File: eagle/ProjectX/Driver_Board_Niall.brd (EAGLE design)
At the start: 100 x 100 mm, 185 parts, among them IC2 NCV78M05BDTRKG, J1 694102303002, U1 TC4427AEOA, U10 TC4427AEOA, U11 TC4427AEOA, U12 TC4427AEOA, U1200 CD74HC4067SM96, U13 TC4427AEOA, U14 TC4427AEOA, U15 TC4427AEOA, U16 TC4427AEOA, U17 TC4427AEOA, U18 TC4427AEOA, U19 TC4427AEOA, U2 TC4427AEOA, U20 TC4427AEOA, U200 ADA4091-2ARZ-RL, U21 TC4427AEOA, U22 TC4427AEOA, U23 TC4427AEOA, U24 TC4427AEOA, U25 TC4427AEOA, U26 TC4427AEOA, U27 TC4427AEOA, U28 TC4427AEOA, U29 TC4427AEOA, U3 TC4427AEOA, U30 TC4427AEOA, U31 TC4427AEOA, U32 TC4427AEOA, U33 TC4427AEOA, U34 TC4427AEOA, U35 TC4427AEOA, U36 TC4427AEOA, U37 TC4427AEOA, U38 TC4427AEOA, U39 TC4427AEOA, U4 TC4427AEOA, U40 TC4427AEOA, U41 TC4427AEOA, U42 TC4427AEOA, U43 TC4427AEOA, U44 TC4427AEOA, U45 TC4427AEOA, U46 TC4427AEOA, U47 TC4427AEOA, U48 TC4427AEOA, U49 TC4427AEOA, U5 TC4427AEOA, U50 TC4427AEOA, U6 TC4427AEOA, U7 TC4427AEOA, U8 TC4427AEOA, U9 TC4427AEOA

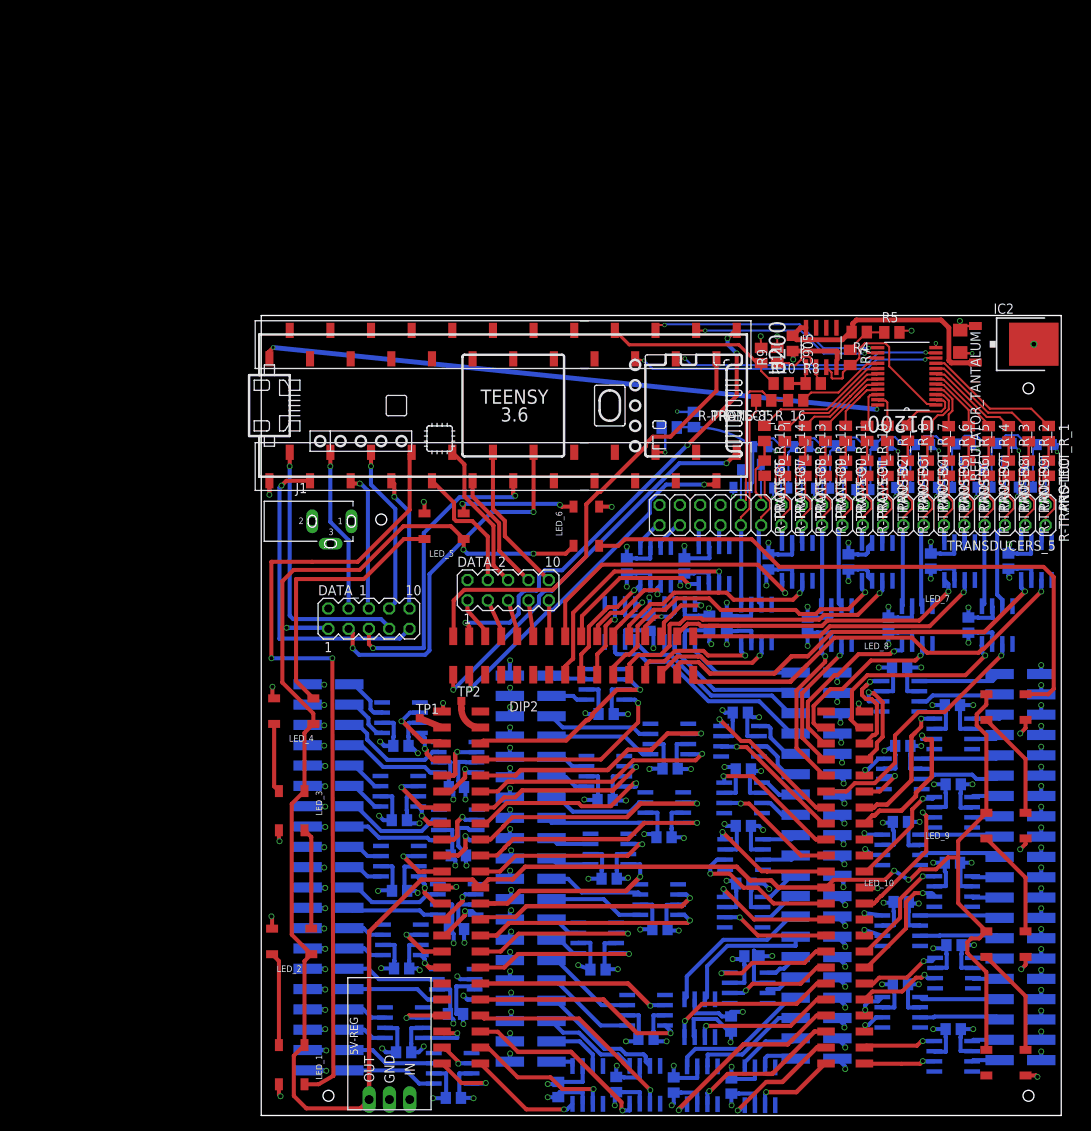
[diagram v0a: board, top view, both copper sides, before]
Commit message: Niall Boards new layout that should slot together
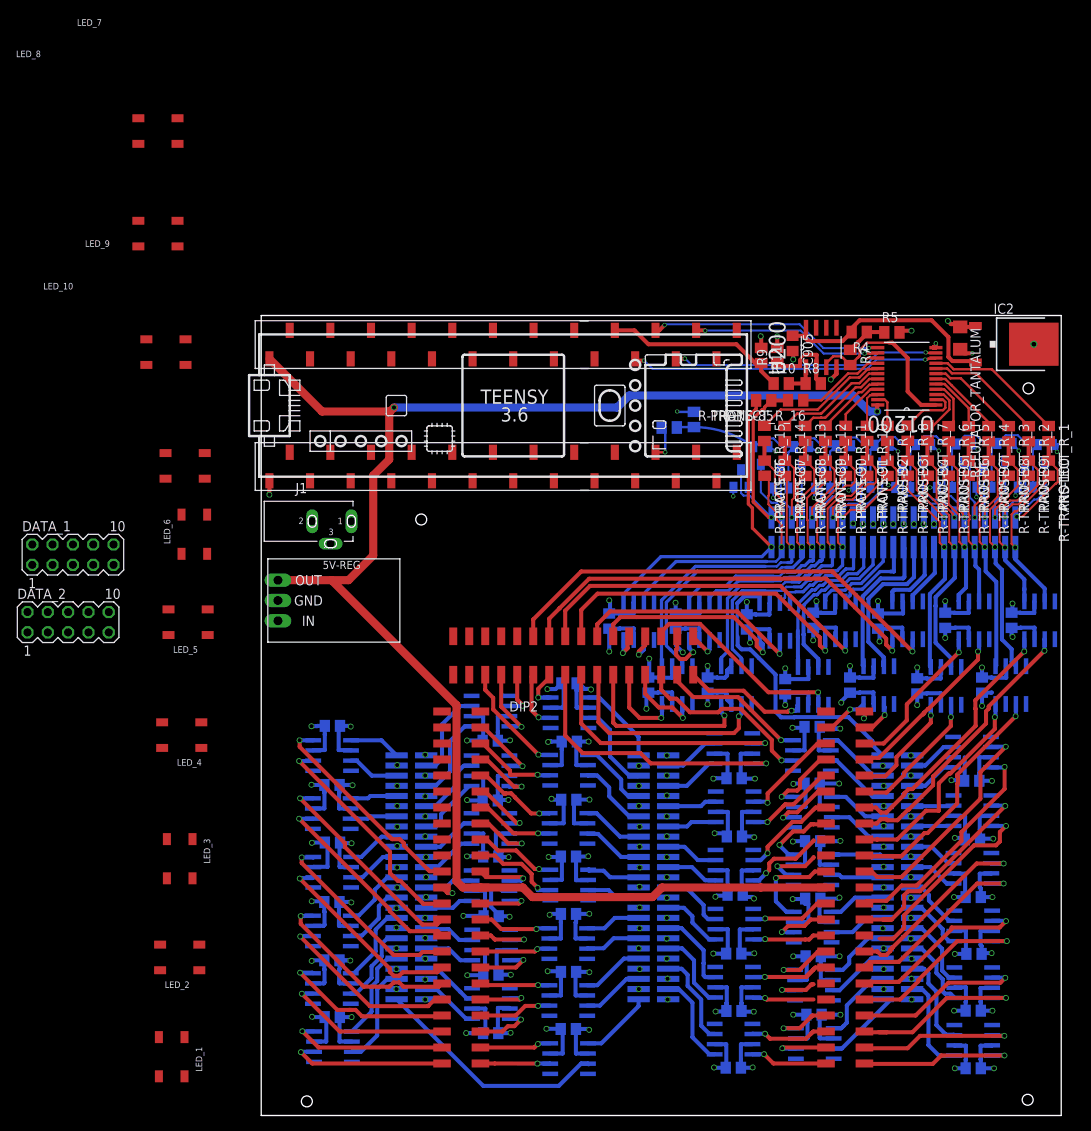
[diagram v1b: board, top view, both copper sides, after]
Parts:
- removed TP1, TP2: TPSTP10SQ, testpad:TP10SQ
- removed TRANSDUCERS_1, TRANSDUCERS_2, TRANSDUCERS_3, TRANSDUCERS_4: 40_PIN_SMD, Parts:40_PIN_SMD
- removed TRANSDUCERS_5: (no value), pinhead:2X20
- added 1, 2, 3, 4: PHB_1MM27_2X25_SNS, _hhn_con_pinhead_box_1mm27:PHB_1MM27_2X25_SNS
- moved LED_8 129.3 mm to (-12.9, 110.2)
- moved LED_9 128.5 mm to (-11.9, 95.4)
- moved LED_7 128.1 mm to (-12.9, 123.1)
- moved LED_10 126.9 mm to (-9.51, 81.2)
- moved 5V-REG 63.9 mm to (2.09, 64.4), turned to 270 degrees
- moved U40 56.3 mm to (72.4, 61.9), turned to 90 degrees
- moved DATA_2 55.1 mm to (-24.1, 61.7)
- moved C40 54.0 mm to (69.0, 61.9), turned to 90 degrees
- moved C12 50.5 mm to (38.5, 54.0), turned to 180 degrees
- moved U38 49.3 mm to (64.2, 61.7), turned to 90 degrees
- moved LED_6 49.0 mm to (-8.36, 72.7)
- moved C38 48.0 mm to (60.7, 61.7), turned to 90 degrees
- moved U12 47.5 mm to (38.5, 50.3), turned to 180 degrees
- moved U20 47.0 mm to (38.5, 7.11), turned to 180 degrees
- moved C29 44.9 mm to (38.5, 46.7), turned to 180 degrees
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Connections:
- removed net N$23: DIP2.8, TP1.TP
- removed net N$24: DIP2.9, TP2.TP
- removed net N$25: DATA_2.9, DIP2.190
- removed net N$26: DATA_2.7, DIP2.193
- removed net N$27: DATA_2.5, DIP2.197
- removed net N$28: DATA_2.1, DIP2.203
- removed net N$29: DATA_2.3, DIP2.200
- net +5V: no longer DATA_1.1
- net 1: now also DIP2.75; no longer DIP2.77
- net 10: now also DIP2.47; no longer DIP2.41
- net 100: now also DIP2.137; no longer DIP2.162
- net 11: now also DIP2.48; no longer DIP2.39
- net 12: now also DIP2.50; no longer DIP2.35
- net 13: now also DIP2.40; no longer DIP2.33
- net 14: now also DIP2.36; no longer DIP2.30
- net 15: now also DIP2.60; no longer DIP2.28
- net 16: now also DIP2.62; no longer DIP2.24
- net 17: now also DIP2.29; no longer DIP2.22
- net 18: now also DIP2.23; no longer DIP2.18
- net 19: now also DIP2.64; no longer DIP2.15
- net 2: now also DIP2.77; no longer DIP2.75
- net 20: now also DIP2.69; no longer DIP2.11
- net 21: now also DIP2.19; no longer DIP2.82
- net 22: now also DIP2.25; no longer DIP2.76
- net 23: now also DIP2.192; no longer DIP2.74
- net 24: now also DIP2.196; no longer DIP2.65
- net 25: now also DIP2.102; no longer DIP2.63
- net 26: now also DIP2.109; no longer DIP2.61
- net 27: now also DIP2.31; no longer DIP2.55
- net 28: now also DIP2.34; no longer DIP2.49
- net 29: now also DIP2.133; no longer DIP2.47
- net 3: now also DIP2.35; no longer DIP2.69
- net 30: now also DIP2.138; no longer DIP2.42
- net 31: now also DIP2.42; no longer DIP2.40
- net 32: now also DIP2.49; no longer DIP2.36
- net 33: now also DIP2.145; no longer DIP2.34
- net 34: now also DIP2.151; no longer DIP2.31
- net 35: now also DIP2.61; no longer DIP2.29
- net 36: now also DIP2.65; no longer DIP2.25
- net 37: now also DIP2.189; no longer DIP2.23
- net 38: now also DIP2.186; no longer DIP2.19
- net 39: now also DIP2.76; no longer DIP2.16
- net 4: now also DIP2.39; no longer DIP2.64
- net 40: now also DIP2.82; no longer DIP2.12
- net 41: now also DIP2.16; no longer DIP2.165
- net 42: now also DIP2.9; no longer DIP2.168
- net 43: now also DIP2.202; no longer DIP2.178
- net 44: now also DIP2.199; no longer DIP2.181
- net 45: now also DIP2.126; no longer DIP2.138
- net 46: now also DIP2.128; no longer DIP2.135
- net 47: now also DIP2.164; no longer DIP2.133
- net 48: now also DIP2.167; no longer DIP2.129
- net 49: now also DIP2.147; no longer DIP2.127
- net 5: now also DIP2.74; no longer DIP2.62
- net 50: now also DIP2.140; no longer DIP2.123
- net 51: now also DIP2.135; no longer DIP2.120
- net 52: now also DIP2.129; no longer DIP2.116
- net 53: now also DIP2.116; no longer DIP2.107
- net 54: now also DIP2.123; no longer DIP2.102
- net 55: now also DIP2.127; no longer DIP2.113
- net 56: now also DIP2.120; no longer DIP2.109
- net 57: now also DIP2.205; no longer DIP2.99
- net 58: now also DIP2.12; no longer DIP2.97
- net 59: now also DIP2.90; no longer DIP2.94
- net 6: now also DIP2.63; no longer DIP2.60
- net 60: now also DIP2.97; no longer DIP2.90
- net 61: now also DIP2.99; no longer DIP2.152
- net 62: now also DIP2.94; no longer DIP2.150
- net 63: now also DIP2.113; no longer DIP2.139
- net 64: now also DIP2.107; no longer DIP2.137
- net 65: now also DIP2.93; no longer DIP2.146
- net 66: now also DIP2.96; no longer DIP2.144
- net 67: now also DIP2.98; no longer DIP2.128
- net 68: now also DIP2.100; no longer DIP2.126
- net 69: now also DIP2.106; no longer DIP2.134
- net 7: now also DIP2.41; no longer DIP2.50
- net 70: now also DIP2.108; no longer DIP2.132
- net 71: now also DIP2.112; no longer DIP2.115
- net 72: now also DIP2.115; no longer DIP2.112
- net 73: now also DIP2.119; no longer DIP2.122
- net 74: now also DIP2.122; no longer DIP2.119
- net 75: now also DIP2.178; no longer DIP2.108
- net 76: now also DIP2.180; no longer DIP2.106
- net 77: now also DIP2.162; no longer DIP2.100
- net 78: now also DIP2.165; no longer DIP2.98
- net 79: now also DIP2.185; no longer DIP2.96
- net 8: now also DIP2.45; no longer DIP2.48
- net 80: now also DIP2.187; no longer DIP2.93
- net 81: now also DIP2.153; no longer DIP2.186
- net 82: now also DIP2.160; no longer DIP2.180
- net 83: now also DIP2.190; no longer DIP2.185
- net 84: now also DIP2.193; no longer DIP2.189
- net 85: now also DIP2.172; no longer DIP2.171
- net 86: now also DIP2.168; no longer DIP2.167
- net 87: now also DIP2.177; no longer DIP2.187
- net 88: now also DIP2.171; no longer DIP2.172
- net 89: now also DIP2.163; no longer DIP2.145
- net 9: now also DIP2.55; no longer DIP2.45
- net 90: now also DIP2.161; no longer DIP2.147
- net 92: now also DIP2.181; no longer DIP2.177
- net 93: now also DIP2.146; no longer DIP2.151
- net 94: now also DIP2.144; no longer DIP2.153
- net 95: now also DIP2.152; no longer DIP2.163
- net 96: now also DIP2.150; no longer DIP2.161
- net 97: now also DIP2.134; no longer DIP2.160
- net 98: now also DIP2.132; no longer DIP2.140
- net 99: now also DIP2.139; no longer DIP2.164
- net FROM_TRANS_100: now also 1.2; no longer TRANSDUCERS_5.1
- net FROM_TRANS_85: now also 1.50; no longer TRANSDUCERS_5.31
- net FROM_TRANS_86: now also 1.48; no longer TRANSDUCERS_5.29
- net FROM_TRANS_87: now also 1.46; no longer TRANSDUCERS_5.27
- net FROM_TRANS_88: now also 1.44; no longer TRANSDUCERS_5.25
- net FROM_TRANS_89: now also 1.42; no longer TRANSDUCERS_5.23
- net FROM_TRANS_90: now also 1.40; no longer TRANSDUCERS_5.21
- net FROM_TRANS_91: now also 1.38; no longer TRANSDUCERS_5.19
- net FROM_TRANS_92: now also 1.36; no longer TRANSDUCERS_5.17
- net FROM_TRANS_93: now also 1.16; no longer TRANSDUCERS_5.15
- net FROM_TRANS_94: now also 1.14; no longer TRANSDUCERS_5.13
- net FROM_TRANS_95: now also 1.12; no longer TRANSDUCERS_5.11
- net FROM_TRANS_96: now also 1.10; no longer TRANSDUCERS_5.9
- net FROM_TRANS_97: now also 1.8; no longer TRANSDUCERS_5.7
- net FROM_TRANS_98: now also 1.6; no longer TRANSDUCERS_5.5
- net FROM_TRANS_99: now also 1.4; no longer TRANSDUCERS_5.3
- net GND: now also 1.18, 1.20, 1.22, 1.24, 1.26, 1.28, 1.30, 1.32, 1.34, 2.10, 2.11, 2.14, 2.15, 2.18, 2.19, 2.2, 2.22, 2.23, 2.26, 2.27, 2.3, 2.30, 2.31, 2.34, 2.35, 2.38, 2.39, 2.42, 2.43, 2.46, 2.47, 2.50, 2.6, 2.7, 3.10, 3.11, 3.14, 3.15, 3.18, 3.19, 3.2, 3.22, 3.23, 3.26, 3.27, 3.3, 3.30, 3.31, 3.34, 3.35, 3.38, 3.39, 3.42, 3.43, 3.46, 3.47, 3.50, 3.6, 3.7, 4.10, 4.11, 4.14, 4.15, 4.18, 4.19, 4.2, 4.22, 4.23, 4.26, 4.27, 4.3, 4.30, 4.31, 4.34, 4.35, 4.38, 4.39, 4.42, 4.43, 4.46, 4.47, 4.50, 4.6, 4.7; no longer DATA_1.2, DATA_2.2, TRANSDUCERS_1.1, TRANSDUCERS_1.11, TRANSDUCERS_1.13, TRANSDUCERS_1.15, TRANSDUCERS_1.17, TRANSDUCERS_1.19, TRANSDUCERS_1.21, TRANSDUCERS_1.23, TRANSDUCERS_1.25, TRANSDUCERS_1.27, TRANSDUCERS_1.29, TRANSDUCERS_1.3, TRANSDUCERS_1.31, TRANSDUCERS_1.33, TRANSDUCERS_1.35, TRANSDUCERS_1.37, TRANSDUCERS_1.39, TRANSDUCERS_1.5, TRANSDUCERS_1.7, TRANSDUCERS_1.9, TRANSDUCERS_2.1, TRANSDUCERS_2.11, TRANSDUCERS_2.13, TRANSDUCERS_2.15, TRANSDUCERS_2.17, TRANSDUCERS_2.19, TRANSDUCERS_2.21, TRANSDUCERS_2.23, TRANSDUCERS_2.25, TRANSDUCERS_2.27, TRANSDUCERS_2.29, TRANSDUCERS_2.3, TRANSDUCERS_2.31, TRANSDUCERS_2.33, TRANSDUCERS_2.35, TRANSDUCERS_2.37, TRANSDUCERS_2.39, TRANSDUCERS_2.5, TRANSDUCERS_2.7, TRANSDUCERS_2.9, TRANSDUCERS_3.1, TRANSDUCERS_3.11, TRANSDUCERS_3.13, TRANSDUCERS_3.15, TRANSDUCERS_3.17, TRANSDUCERS_3.19, TRANSDUCERS_3.21, TRANSDUCERS_3.23, TRANSDUCERS_3.25, TRANSDUCERS_3.27, TRANSDUCERS_3.29, TRANSDUCERS_3.3, TRANSDUCERS_3.31, TRANSDUCERS_3.33, TRANSDUCERS_3.35, TRANSDUCERS_3.37, TRANSDUCERS_3.39, TRANSDUCERS_3.5, TRANSDUCERS_3.7, TRANSDUCERS_3.9, TRANSDUCERS_4.1, TRANSDUCERS_4.11, TRANSDUCERS_4.13, TRANSDUCERS_4.15, TRANSDUCERS_4.17, TRANSDUCERS_4.19, TRANSDUCERS_4.21, TRANSDUCERS_4.23, TRANSDUCERS_4.25, TRANSDUCERS_4.27, TRANSDUCERS_4.29, TRANSDUCERS_4.3, TRANSDUCERS_4.31, TRANSDUCERS_4.33, TRANSDUCERS_4.35, TRANSDUCERS_4.37, TRANSDUCERS_4.39, TRANSDUCERS_4.5, TRANSDUCERS_4.7, TRANSDUCERS_4.9, TRANSDUCERS_5.33, TRANSDUCERS_5.35, TRANSDUCERS_5.37, TRANSDUCERS_5.39
- net TEENSY_DATA_0: no longer DATA_1.7
- net TEENSY_DATA_1: no longer DATA_1.9
- net TEENSY_DATA_10: no longer DATA_2.10
- net TEENSY_DATA_11: no longer DATA_1.5
- net TEENSY_DATA_12: no longer DATA_1.3
- net TEENSY_DATA_2: no longer DATA_1.4
- net TEENSY_DATA_3: no longer DATA_1.6
- net TEENSY_DATA_31: no longer DIP2.3
- net TEENSY_DATA_32: no longer DIP2.5
- net TEENSY_DATA_33: no longer DIP2.2
- net TEENSY_DATA_34: no longer DIP2.4
- net TEENSY_DATA_4: no longer DATA_1.8
- net TEENSY_DATA_5: no longer DATA_1.10
- net TEENSY_DATA_7: no longer DATA_2.4
- net TEENSY_DATA_8: no longer DATA_2.6
- net TEENSY_DATA_9: no longer DATA_2.8
- net TO_TRAN_1: now also 4.9; no longer TRANSDUCERS_1.2
- net TO_TRAN_10: now also 4.16; no longer TRANSDUCERS_1.20
- net TO_TRAN_100: now also 1.1; no longer TRANSDUCERS_5.2
- net TO_TRAN_11: now also 4.33; no longer TRANSDUCERS_1.22
- net TO_TRAN_12: now also 4.29; no longer TRANSDUCERS_1.24
- net TO_TRAN_13: now also 4.20; no longer TRANSDUCERS_1.26
- net TO_TRAN_14: now also 4.24; no longer TRANSDUCERS_1.28
- net TO_TRAN_15: now also 4.25; no longer TRANSDUCERS_1.30
- net TO_TRAN_16: now also 4.21; no longer TRANSDUCERS_1.32
- net TO_TRAN_17: now also 4.28; no longer TRANSDUCERS_1.34
- net TO_TRAN_18: now also 4.32; no longer TRANSDUCERS_1.36
- net TO_TRAN_19: now also 4.17; no longer TRANSDUCERS_1.38
- net TO_TRAN_2: now also 4.5; no longer TRANSDUCERS_1.4
- net TO_TRAN_20: now also 4.13; no longer TRANSDUCERS_1.40
- net TO_TRAN_21: now also 3.33; no longer TRANSDUCERS_2.2
- net TO_TRAN_22: now also 3.29; no longer TRANSDUCERS_2.4
- net TO_TRAN_23: now also 3.49; no longer TRANSDUCERS_2.6
- net TO_TRAN_24: now also 3.45; no longer TRANSDUCERS_2.8
- net TO_TRAN_25: now also 3.12; no longer TRANSDUCERS_2.10
- net TO_TRAN_26: now also 3.16; no longer TRANSDUCERS_2.12
- net TO_TRAN_27: now also 3.25; no longer TRANSDUCERS_2.14
- net TO_TRAN_28: now also 3.21; no longer TRANSDUCERS_2.16
- net TO_TRAN_29: now also 3.28; no longer TRANSDUCERS_2.18
- net TO_TRAN_3: now also 4.49; no longer TRANSDUCERS_1.6
- net TO_TRAN_30: now also 3.32; no longer TRANSDUCERS_2.20
- net TO_TRAN_31: now also 3.17; no longer TRANSDUCERS_2.22
- net TO_TRAN_32: now also 3.13; no longer TRANSDUCERS_2.24
- net TO_TRAN_33: now also 3.36; no longer TRANSDUCERS_2.26
- net TO_TRAN_34: now also 3.40; no longer TRANSDUCERS_2.28
- net TO_TRAN_35: now also 3.9; no longer TRANSDUCERS_2.30
- net TO_TRAN_36: now also 3.5; no longer TRANSDUCERS_2.32
- net TO_TRAN_37: now also 3.44; no longer TRANSDUCERS_2.34
- net TO_TRAN_38: now also 3.48; no longer TRANSDUCERS_2.36
- net TO_TRAN_39: now also 3.1; no longer TRANSDUCERS_2.38
- net TO_TRAN_4: now also 4.45; no longer TRANSDUCERS_1.8
- net TO_TRAN_40: now also 4.1; no longer TRANSDUCERS_2.40
- net TO_TRAN_41: now also 4.36; no longer TRANSDUCERS_3.2
- net TO_TRAN_42: now also 4.40; no longer TRANSDUCERS_3.4
- net TO_TRAN_43: now also 4.44; no longer TRANSDUCERS_3.6
- net TO_TRAN_44: now also 4.48; no longer TRANSDUCERS_3.8
- net TO_TRAN_45: now also 2.44; no longer TRANSDUCERS_3.10
- net TO_TRAN_46: now also 2.48; no longer TRANSDUCERS_3.12
- net TO_TRAN_47: now also 2.45; no longer TRANSDUCERS_3.14
- net TO_TRAN_48: now also 2.41; no longer TRANSDUCERS_3.16
- net TO_TRAN_49: now also 2.37; no longer TRANSDUCERS_3.18
- net TO_TRAN_5: now also 4.4; no longer TRANSDUCERS_1.10
- net TO_TRAN_50: now also 2.33; no longer TRANSDUCERS_3.20
- net TO_TRAN_51: now also 2.29; no longer TRANSDUCERS_3.22
- net TO_TRAN_52: now also 2.25; no longer TRANSDUCERS_3.24
- net TO_TRAN_53: now also 3.20; no longer TRANSDUCERS_3.26
- net TO_TRAN_54: now also 3.24; no longer TRANSDUCERS_3.28
- net TO_TRAN_55: now also 2.21; no longer TRANSDUCERS_3.30
- net TO_TRAN_56: now also 2.17; no longer TRANSDUCERS_3.32
- net TO_TRAN_57: now also 3.41; no longer TRANSDUCERS_3.34
- net TO_TRAN_58: now also 3.37; no longer TRANSDUCERS_3.36
- net TO_TRAN_59: now also 3.4; no longer TRANSDUCERS_3.38
- net TO_TRAN_6: now also 4.8; no longer TRANSDUCERS_1.12
- net TO_TRAN_60: now also 3.8; no longer TRANSDUCERS_3.40
- net TO_TRAN_61: now also 2.5; no longer TRANSDUCERS_4.2
- net TO_TRAN_62: now also 2.1; no longer TRANSDUCERS_4.4
- net TO_TRAN_63: now also 2.13; no longer TRANSDUCERS_4.6
- net TO_TRAN_64: now also 2.9; no longer TRANSDUCERS_4.8
- net TO_TRAN_65: now also 2.4; no longer TRANSDUCERS_4.10
- net TO_TRAN_66: now also 2.8; no longer TRANSDUCERS_4.12
- net TO_TRAN_67: now also 2.12; no longer TRANSDUCERS_4.14
- net TO_TRAN_68: now also 2.16; no longer TRANSDUCERS_4.16
- net TO_TRAN_69: now also 2.20; no longer TRANSDUCERS_4.18
- net TO_TRAN_7: now also 4.41; no longer TRANSDUCERS_1.14
- net TO_TRAN_70: now also 2.24; no longer TRANSDUCERS_4.20
- net TO_TRAN_71: now also 2.28; no longer TRANSDUCERS_4.22
- net TO_TRAN_72: now also 2.32; no longer TRANSDUCERS_4.24
- net TO_TRAN_73: now also 2.36; no longer TRANSDUCERS_4.26
- net TO_TRAN_74: now also 2.40; no longer TRANSDUCERS_4.28
- net TO_TRAN_75: now also 2.49; no longer TRANSDUCERS_4.30
- net TO_TRAN_76: now also 1.33; no longer TRANSDUCERS_4.32
- net TO_TRAN_77: now also 1.31; no longer TRANSDUCERS_4.34
- net TO_TRAN_78: now also 1.29; no longer TRANSDUCERS_4.36
- net TO_TRAN_79: now also 1.27; no longer TRANSDUCERS_4.38
- net TO_TRAN_8: now also 4.37; no longer TRANSDUCERS_1.16
- net TO_TRAN_80: now also 1.25; no longer TRANSDUCERS_4.40
- net TO_TRAN_81: now also 1.23; no longer TRANSDUCERS_5.40
- net TO_TRAN_82: now also 1.21; no longer TRANSDUCERS_5.38
- net TO_TRAN_83: now also 1.19; no longer TRANSDUCERS_5.36
- net TO_TRAN_84: now also 1.17; no longer TRANSDUCERS_5.34
- net TO_TRAN_85: now also 1.49; no longer TRANSDUCERS_5.32
- net TO_TRAN_86: now also 1.47; no longer TRANSDUCERS_5.30
- net TO_TRAN_87: now also 1.45; no longer TRANSDUCERS_5.28
- net TO_TRAN_88: now also 1.43; no longer TRANSDUCERS_5.26
- net TO_TRAN_89: now also 1.41; no longer TRANSDUCERS_5.24
- net TO_TRAN_9: now also 4.12; no longer TRANSDUCERS_1.18
- net TO_TRAN_90: now also 1.39; no longer TRANSDUCERS_5.22
- net TO_TRAN_91: now also 1.37; no longer TRANSDUCERS_5.20
- net TO_TRAN_92: now also 1.35; no longer TRANSDUCERS_5.18
- net TO_TRAN_93: now also 1.15; no longer TRANSDUCERS_5.16
- net TO_TRAN_94: now also 1.13; no longer TRANSDUCERS_5.14
- net TO_TRAN_95: now also 1.11; no longer TRANSDUCERS_5.12
- net TO_TRAN_96: now also 1.9; no longer TRANSDUCERS_5.10
- net TO_TRAN_97: now also 1.7; no longer TRANSDUCERS_5.8
- net TO_TRAN_98: now also 1.5; no longer TRANSDUCERS_5.6
- net TO_TRAN_99: now also 1.3; no longer TRANSDUCERS_5.4
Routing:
- net +5V: track 361.9 -> 205.0 mm, vias 7 -> 2
- net GND: track 499.3 -> 351.7 mm, vias 170 -> 163
- net N$22: track 103.0 -> 0.00 mm, vias 2 -> 0
- net N$18: track 76.9 -> 0.00 mm
- net TEENSY_DATA_33: track 59.0 -> 0.00 mm, vias 4 -> 0
- net TEENSY_DATA_34: track 56.2 -> 0.00 mm
- net TEENSY_DATA_32: track 50.2 -> 0.00 mm, vias 2 -> 0
- net TEENSY_DATA_12: track 46.1 -> 0.00 mm, vias 2 -> 0
- net TEENSY_DATA_31: track 44.2 -> 0.00 mm, vias 2 -> 0
- net TEENSY_DATA_1: track 40.0 -> 0.00 mm, vias 1 -> 0
- net TO_TRAN_75: track 3.37 -> 42.4 mm
- net TEENSY_DATA_11: track 38.7 -> 0.00 mm, vias 2 -> 0
- net 80: track 8.90 -> 44.3 mm
- net N$16: track 33.9 -> 0.00 mm
- net TEENSY_DATA_0: track 33.7 -> 0.00 mm, vias 1 -> 0
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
